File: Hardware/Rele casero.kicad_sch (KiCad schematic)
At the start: 15 parts, among them J1 Screw_Terminal_01x02, J2 Screw_Terminal_01x02, K1 SANYOU_SRD_Form_C, Q1 PN2222A, U1 ESP32C3-SUPERMINI, U2 4N25, U4 SMTS-102

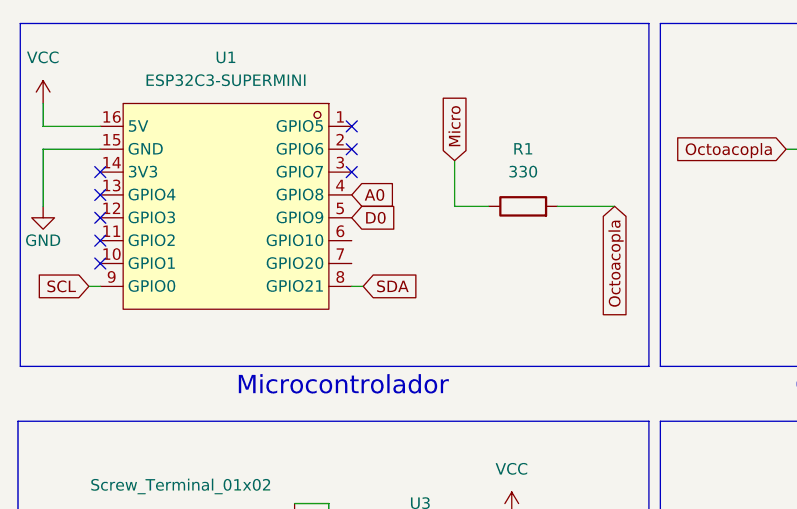
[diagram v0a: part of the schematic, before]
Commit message: Add files via upload
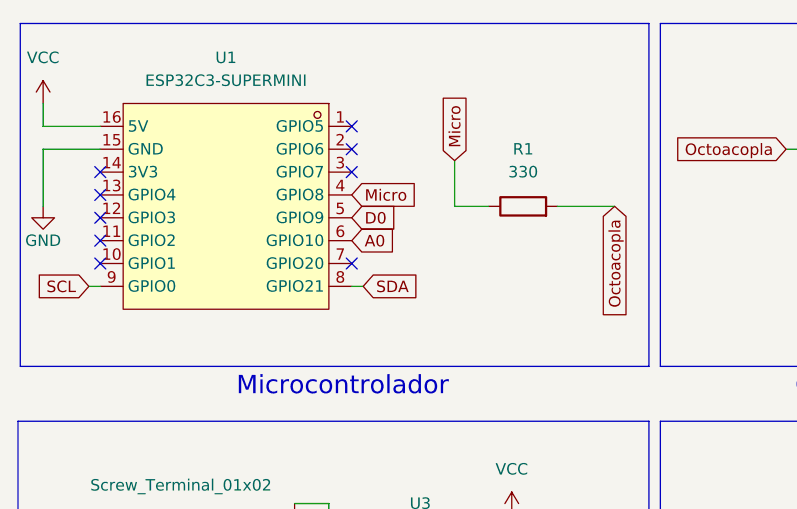
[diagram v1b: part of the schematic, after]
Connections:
- net A0: now also U1.6 (GPIO10); no longer U1.4 (GPIO8)
- net Micro: now also U1.4 (GPIO8)
- no-connect marks 11 -> 12
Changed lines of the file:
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@@
+	)
+	(no_connect
+		(at 50.8 43.18)
+	)
+	(no_connect
+		(at 50.8 33.02)
 	)
 	(no_connect
@@
 	)
 	(no_connect
-		(at 50.8 33.02)
-	)
-	(no_connect
 		(at 22.86 35.56)
 	)
@@
 	(global_label "A0"
 		(shape input)
+		(at 50.8 40.64 0)
+		(fields_autoplaced yes)
+		(effects
+			(font
+				(size 1.27 1.27)
+			)
+			(justify left)
+		)
+		(property "Intersheetrefs" "${INTERSHEET_REFS}"
+			(at 56.0833 40.64 0)
+			(hide yes)
+			(show_name no)
+			(do_not_autoplace no)
+			(effects
+				(font
+					(size 1.27 1.27)
+				)
+				(justify left)
+			)
+		)
+	)
+	(global_label "Micro"
+		(shape input)
 		(at 50.8 35.56 0)
 		(fields_autoplaced yes)
@@
 		)
 		(property "Intersheetrefs" "${INTERSHEET_REFS}"
-			(at 56.0833 35.56 0)
-			(hide yes)
-			(show_name no)
+			(at 58.8652 35.56 0)
+			(hide yes)
+			(show_name no)

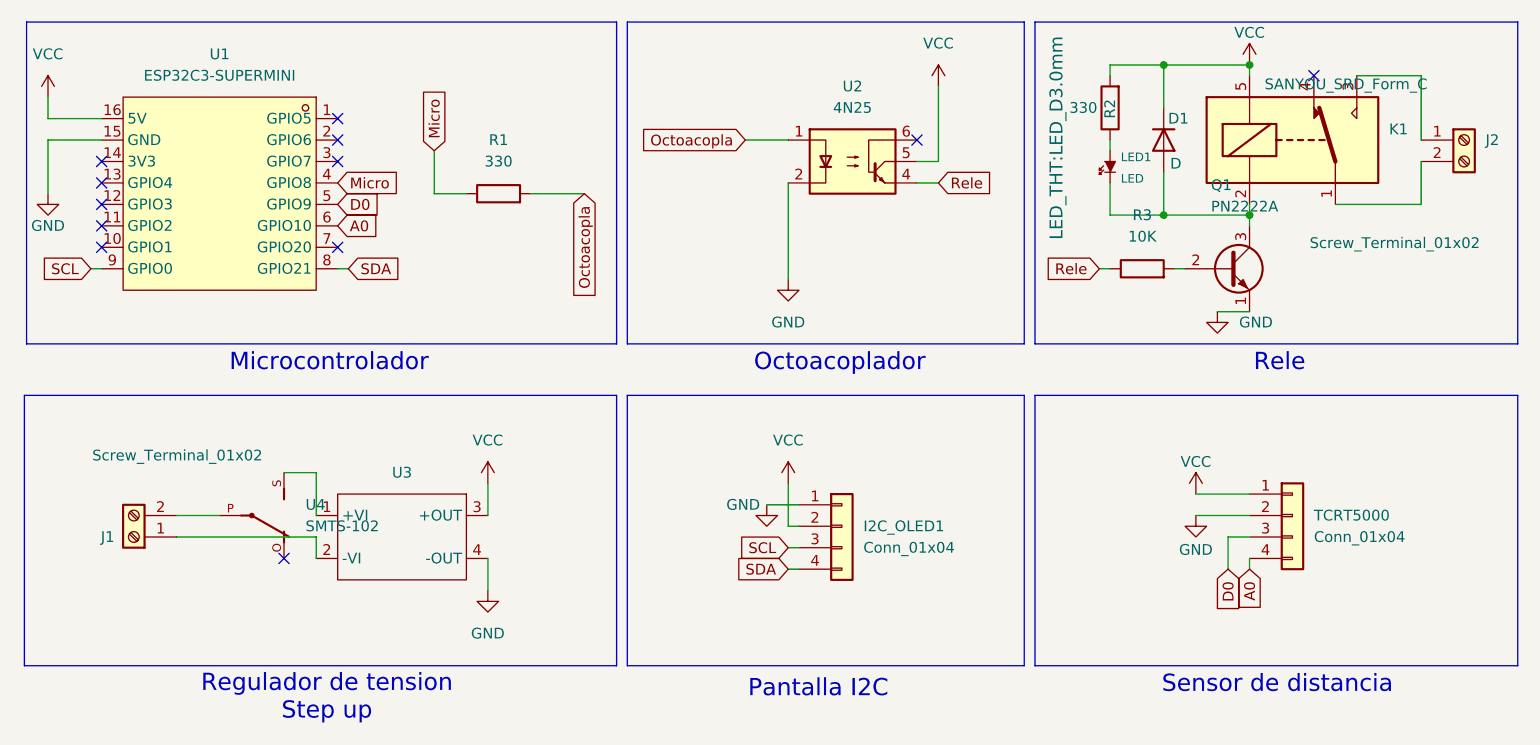
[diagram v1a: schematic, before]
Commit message: Add files via upload
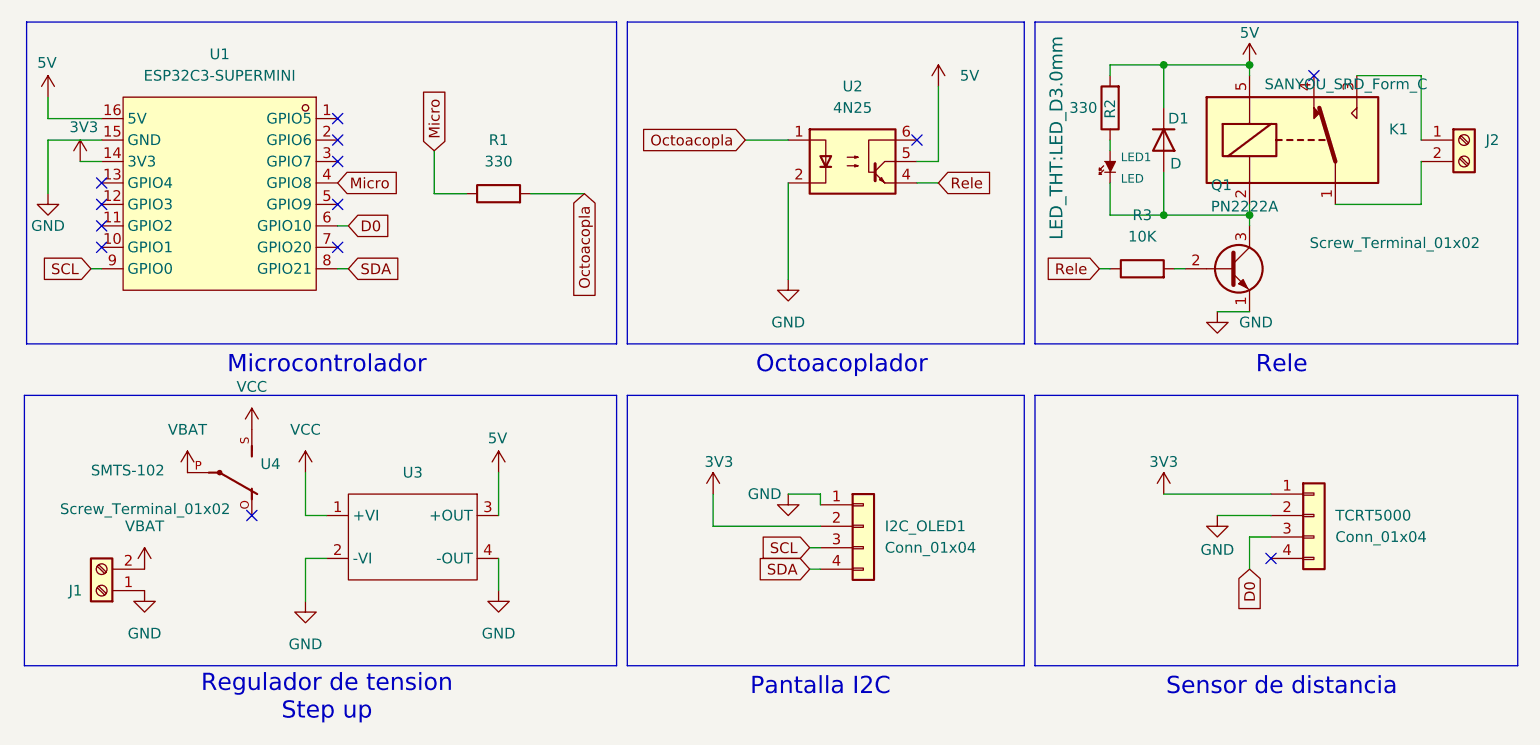
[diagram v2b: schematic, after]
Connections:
- net D0: now also U1.6 (GPIO10); no longer U1.5 (GPIO9)
- net GND: now also J1.1 (Pin_1), U3.2 (-VI)
- net VCC: now also U3.1 (+VI), U4.S; no longer D1.1 (K), I2C_OLED1.2 (Pin_2), K1.5, R2.2, TCRT5000.1 (Pin_1), U1.16 (5V), U2.5, U3.3 (+OUT)
- net VBAT: now reaches J1.2 (Pin_2), U4.P
- net 3V3: now reaches U1.14 (3V3)
- net 3V3: now also I2C_OLED1.2 (Pin_2), TCRT5000.1 (Pin_1)
- net A0: no longer names the net of TCRT5000.4 (Pin_4)
- net A0: no longer U1.6 (GPIO10)
- new net 5V: D1.1 (K), K1.5, R2.2, U1.16 (5V), U2.5, U3.3 (+OUT)
- no-connect marks 12 -> 13
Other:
- moved on the sheet: I2C_OLED1, J1, TCRT5000, U3, U4
